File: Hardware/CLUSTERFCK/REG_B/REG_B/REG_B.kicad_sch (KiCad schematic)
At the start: 20 parts, among them U16 74LS173, U17 74LS173

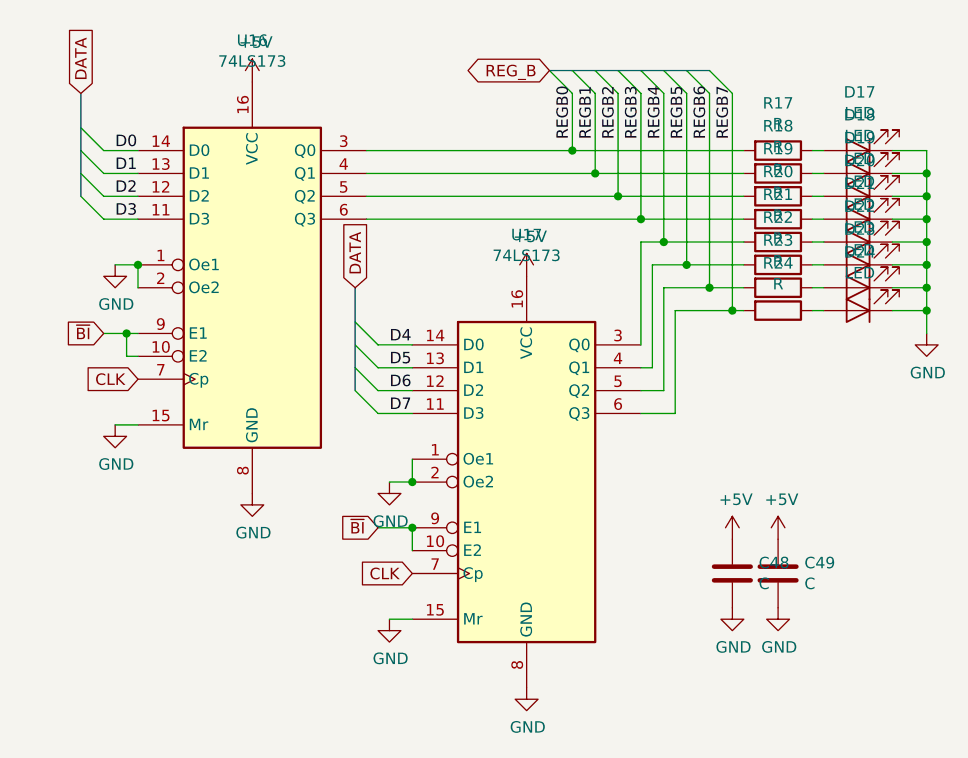
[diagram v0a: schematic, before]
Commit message: 17 | 1h | beautifyed several scematics
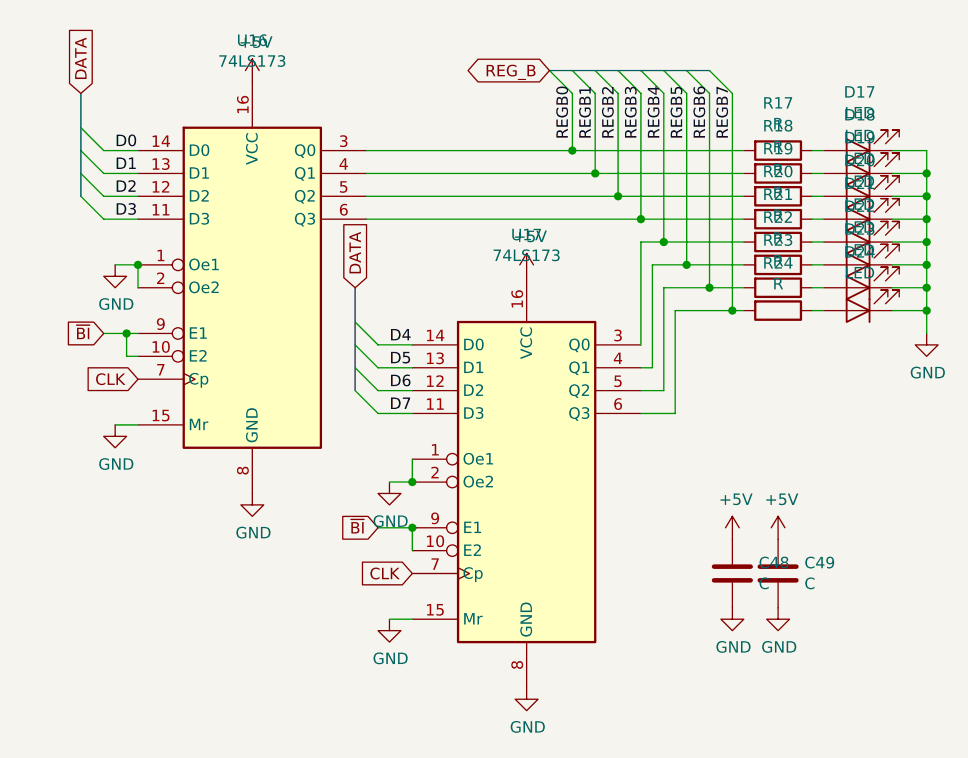
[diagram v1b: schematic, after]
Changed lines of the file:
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@@
   (title_block
     (title "REG_B")
-    (date "2020-10-06")
+    (date "2020-10-10")
     (rev "1")
     (company "Wilhelm-Maybach-Schule Heilbronn")
+    (comment 1 "Leon Hellmich")
   )
   (junction (at 100.965 96.52) (diameter 0) (color 0 0 0 0))
@@
     (stroke (width 0) (type solid) (color 0 0 0 0))
   )
-  (bus (pts (xy 126.365 91.44) (xy 126.365 95.25))
-    (stroke (width 0) (type solid) (color 0 0 0 0))
-  )
-  (bus (pts (xy 126.365 95.25) (xy 126.365 100.33))
-    (stroke (width 0) (type solid) (color 0 0 0 0))
-  )
-  (bus (pts (xy 126.365 100.33) (xy 126.365 102.87))
-    (stroke (width 0) (type solid) (color 0 0 0 0))
-  )
+  (bus (pts (xy 126.365 91.44) (xy 126.365 97.79))
+    (stroke (width 0) (type solid) (color 0 0 0 0))
+  )
+  (bus (pts (xy 126.365 97.79) (xy 126.365 102.87))
+    (stroke (width 0) (type solid) (color 0 0 0 0))
+  )
